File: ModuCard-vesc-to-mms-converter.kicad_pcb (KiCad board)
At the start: 2 copper layers, 60 x 94.5 mm, 42 parts, among them J1 RJ45_LED_Shielded, J2 RJ45_LED_Shielded, J3 Conn_01x04, J4 Conn_01x05, J5 VCC_IN, SW1 SW_DIP_x02, U1 CH334R, Y1 12Mhz

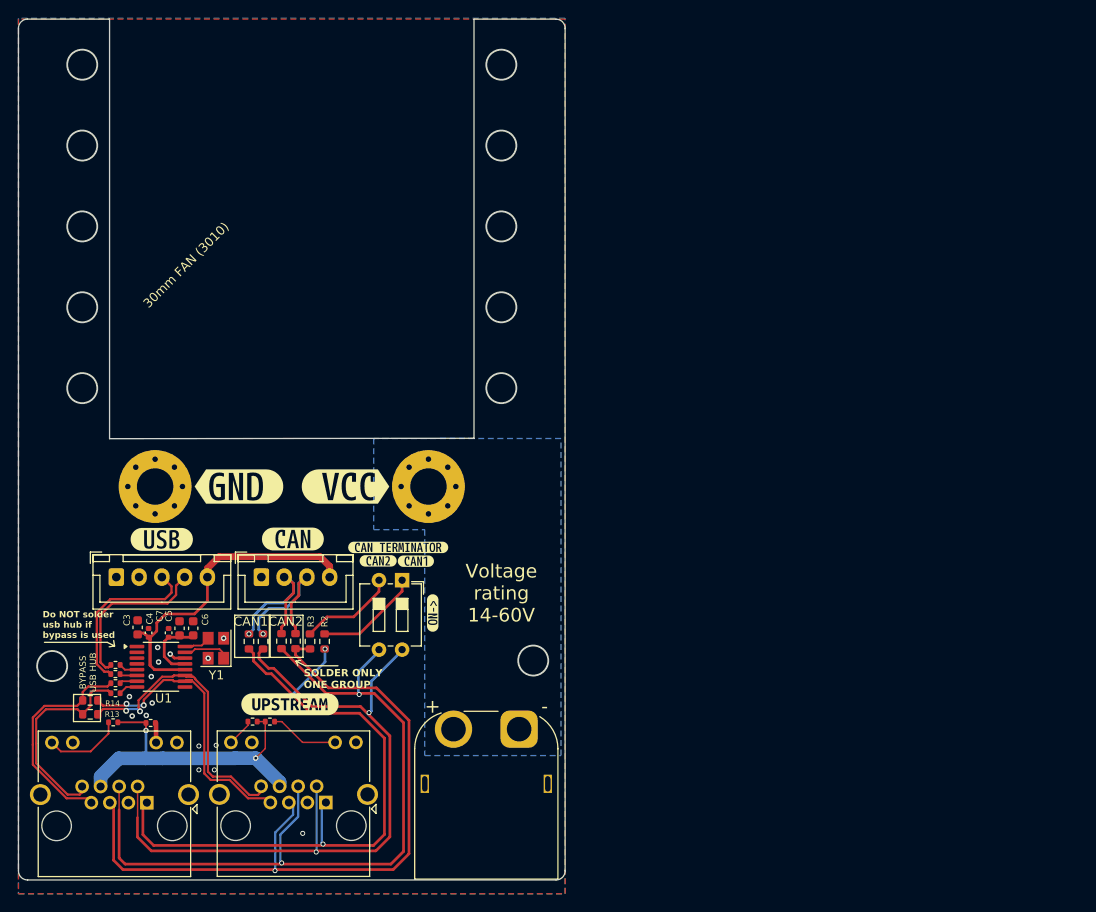
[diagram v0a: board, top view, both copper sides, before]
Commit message: rev v3 tiny
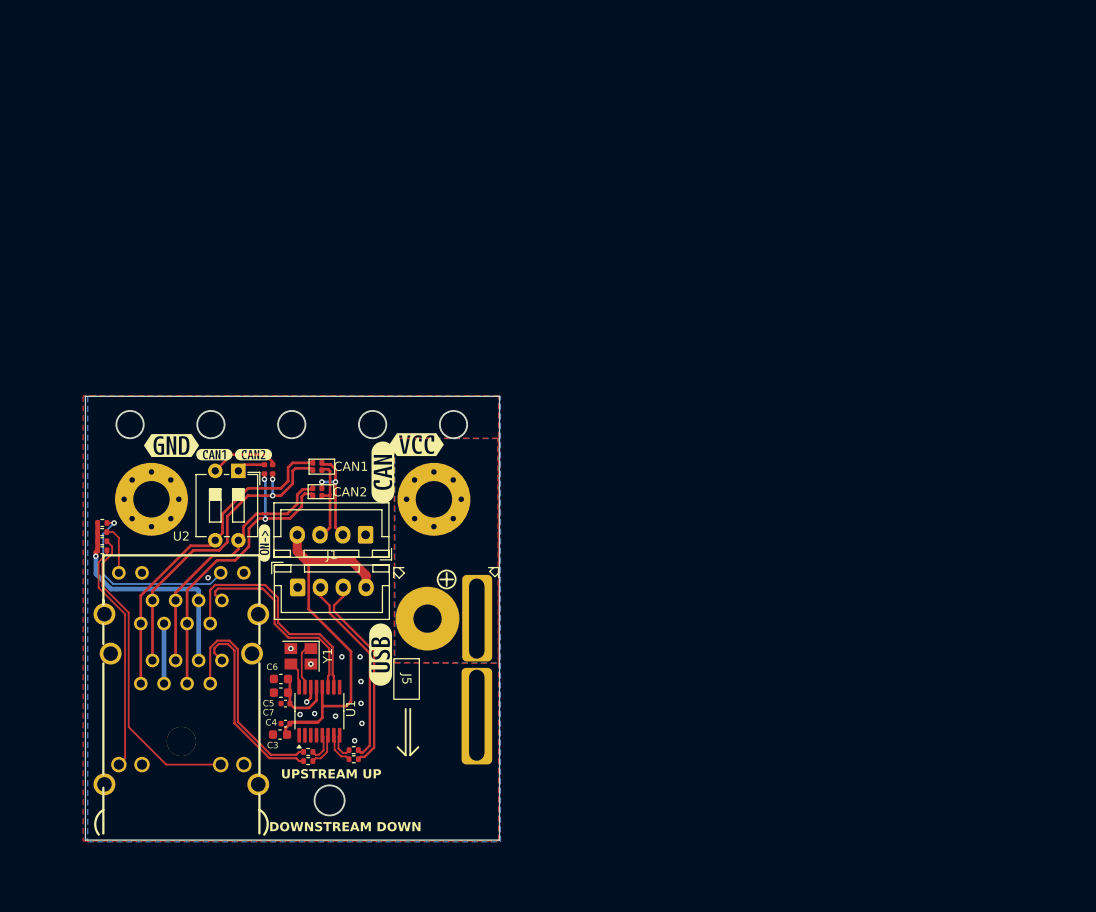
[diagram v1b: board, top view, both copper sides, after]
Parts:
- removed J2: RJ45_LED_Shielded, Connector_RJ:RJ45_Amphenol_RJHSE538X
- removed J4: Conn_01x05, Connector_JST:JST_XH_B5B-XH-A_1x05_P2.50mm_Vertical
- removed R13, R14, R8: 0R, Resistor_SMD:R_0603_1608Metric
- removed R17, R18: 1k, Resistor_SMD:R_0402_1005Metric
- removed R3: 120R, Resistor_SMD:R_0603_1608Metric
- removed kibuzzard-673147F0: G***, kibuzzard-673147F0
- removed kibuzzard-67314807: G***, kibuzzard-67314807
- removed kibuzzard-674E462A: G***, kibuzzard-674E462A
- removed kibuzzard-6754762D: G***, kibuzzard-6754762D
- removed kibuzzard-675D9C67: G***, kibuzzard-675D9C67
- removed kibuzzard-68D8378B: G***, kibuzzard-68D8378B
- removed kibuzzard-68D83794: G***, kibuzzard-68D83794
- added R15: 1k, Resistor_SMD:R_0402_1005Metric, F.Cu at (89.2, 111.3)
- added R16: 1k, Resistor_SMD:R_0402_1005Metric, F.Cu at (89.2, 112.3)
- added R19: 1k, Resistor_SMD:R_0402_1005Metric, F.Cu at (89.2, 109.3)
- added R20: 1k, Resistor_SMD:R_0402_1005Metric, F.Cu at (89.2, 110.3)
- added U2: XDRJ-1609-002, rj45:RJ45-TH_XDRJ-1609-002, F.Cu at (97.9, 126.4)
- added kibuzzard-68DAF865: G***, kibuzzard-68DAF865, F.Cu at (123.7, 100.7)
- added kibuzzard-68DAF86F: G***, kibuzzard-68DAF86F, F.Cu at (96.8, 100.8)
- added kibuzzard-68DB0050: G***, kibuzzard-68DB0050, F.Cu at (120.0, 103.8)
- J1: value RJ45_LED_Shielded -> Conn_01x04; footprint Connector_RJ:RJ45_Amphenol_RJHSE538X -> Connector_JST:JST_XH_B4B-XH-A_1x04_P2.50mm_Vertical
- J5: footprint Connector_AMASS:AMASS_XT60PW-M_1x02_P7.20mm_Horizontal -> lib:XT60-RightAngle-Adapter
- R1, R4: value 1k -> 0Ω; footprint Resistor_SMD:R_0402_1005Metric -> PCM_JLCPCB:R_0402
- R2: value 120R -> 120Ω; footprint Resistor_SMD:R_0603_1608Metric -> PCM_JLCPCB:R_0402
- R5, R6: value 0R -> 0Ω; footprint Resistor_SMD:R_0603_1608Metric -> PCM_JLCPCB:R_0402
- R7: value 0R -> 120Ω; footprint Resistor_SMD:R_0603_1608Metric -> PCM_JLCPCB:R_0402
- moved R4 36.2 mm to (112.8, 102.7), turned to 0 degrees
- moved R1 28.1 mm to (112.8, 103.5)
- moved R11 27.4 mm to (116.8, 135.2), turned to 0 degrees
- moved kibuzzard-674E4620 27.1 mm to (119.8, 123.8), turned to 90 degrees
- moved R12 26.9 mm to (116.8, 134.2), turned to 180 degrees
- moved kibuzzard-675D9C73 25.0 mm to (101.5, 101.8)
- moved J1 23.8 mm to (110.7, 116.4), turned to 0 degrees
- moved R10 23.2 mm to (111.8, 135.4)
- moved R9 23.2 mm to (111.8, 134.4)
- moved SW1 21.6 mm to (104.1, 103.6)
- moved kibuzzard-675D9CCD 20.0 mm to (107.0, 111.5)
- moved R2 19.7 mm to (107.9, 103.4)
- moved C3 19.6 mm to (108.7, 132.5), turned to 0 degrees
- moved R7 19.0 mm to (107.0, 103.4)
- moved U1 18.1 mm to (113.0, 130.0), turned to 90 degrees
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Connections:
- J1 pad 1: /CAN/CAN1- -> GND
- J1 pad 2: /CAN/CAN1+ -> /USB/USB_VESC_D+
- J1 pad 3: GND -> /USB/USB_VESC_D-
- J1 pad 4: /CAN/CAN2- -> +5V
- J5 pad 1: GND -> VCC
- J5 pad 2: VCC -> GND
- R1 pad 1: +12V -> /CAN/CAN1+
- R1 pad 2: Net-(J1-Pad10) -> /CAN/CAN+
- R10 pad 1: /USB/USB_VESC_D+ -> USB_DOWNSTREAM_D+
- R11 pad 2: USB_DOWNSTREAM_D- -> /USB/USB_VESC_D-
- R12 pad 1: USB_DOWNSTREAM_D+ -> /USB/USB_VESC_D+
- R2 pad 1: /CAN/CAN1- -> /CAN/CAN1+
- R4 pad 1: +12V -> /CAN/CAN1-
- R4 pad 2: Net-(J2-Pad12) -> /CAN/CAN-
- R5 pad 1: /CAN/CAN2+ -> /CAN/CAN+
- R5 pad 2: /CAN/CAN+ -> /CAN/CAN2+
- R6 pad 1: /CAN/CAN+ -> /CAN/CAN-
- R6 pad 2: /CAN/CAN1+ -> /CAN/CAN2-
- R7 pad 1: /CAN/CAN2- -> /CAN/CAN2+
- R7 pad 2: /CAN/CAN- -> Net-(R7-Pad2)
- R9 pad 1: /USB/USB_VESC_D- -> USB_DOWNSTREAM_D-
- SW1 pad 1: Net-(R2-Pad2) -> Net-(R7-Pad2)
- SW1 pad 2: Net-(R3-Pad2) -> Net-(R2-Pad2)
- SW1 pad 3: /CAN/CAN2- -> /CAN/CAN1-
- SW1 pad 4: /CAN/CAN1+ -> /CAN/CAN2-
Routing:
- net /CAN/CAN2-: track 86.0 -> 29.5 mm, vias 2 -> 0
- net /CAN/CAN2+: track 80.9 -> 35.3 mm, vias 1 -> 2
- net /CAN/CAN1+: track 80.4 -> 35.7 mm
- net /CAN/CAN1-: track 72.7 -> 36.7 mm, vias 3 -> 0
- net Net-(R15-Pad1): track 0.00 -> 34.1 mm
- net Net-(R16-Pad1): track 0.00 -> 25.4 mm
- net Net-(R19-Pad1): track 0.00 -> 20.8 mm, vias 0 -> 1
- net Net-(R3-Pad2): track 10.7 -> 0.00 mm
- net USB_UPSTREAM_D+: track 33.1 -> 22.5 mm, vias 2 -> 0
- net +12V: track 35.4 -> 25.4 mm, vias 2 -> 1
- net Net-(J2-Pad12): track 8.66 -> 0.00 mm
- net Net-(J1-Pad10): track 7.59 -> 0.00 mm
- net /CAN/CAN+: track 17.1 -> 9.64 mm, vias 1 -> 0
- net GND: track 1.81 -> 8.40 mm, vias 15 -> 13
- net USB_UPSTREAM_D-: track 32.5 -> 26.2 mm, vias 2 -> 0
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- added copper zone on F.Cu, net VCC
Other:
- board size 60 x 94.5 mm -> 45.5 x 48.7 mm
- board text added: "DOWNSTREAM DOWN"
- board text added: "UPSTREAM UP"
- board text removed: "30mm FAN (3010)"
- board text removed: "BYPASS USB HUB"
- board text removed: "Do NOT solder usb hub if bypass is used"
- board text removed: "R13"
- board text removed: "R14"
- board text removed: "SOLDER ONLY ONE GROUP"
- board text removed: "USB BYPASS BLOCK DIAGRAM"
- board text removed: "USB HUB"
- board text removed: "USB IN"
- board text removed: "USB OUT"

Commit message: rev 1
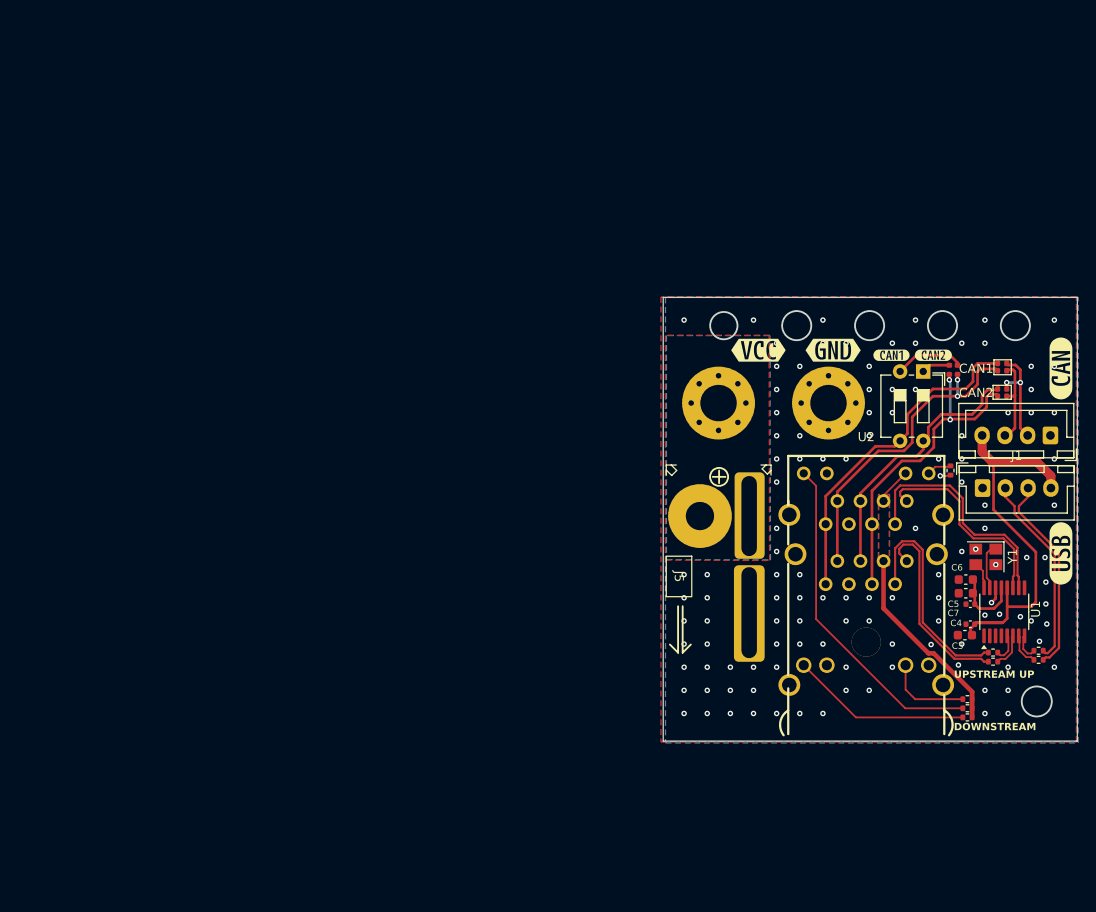
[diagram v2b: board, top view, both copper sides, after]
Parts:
- removed kibuzzard-675D9CCD: G***, kibuzzard-675D9CCD
- moved R20 96.9 mm to (184.2, 129.6), turned to 0 degrees
- moved R16 96.7 mm to (184.2, 130.6), turned to 0 degrees
- moved R15 96.5 mm to (184.2, 128.6), turned to 0 degrees
- moved R19 93.3 mm to (182.3, 103.5), turned to -90 degrees
- moved J3 76.0 mm to (193.3, 99.7)
- moved R7 76.0 mm to (182.2, 92.5)
- moved U1 76.0 mm to (188.2, 119.1)
- moved U2 76.0 mm to (173.0, 115.5)
- moved Y1 76.0 mm to (186.2, 113.0)
- moved C3 76.0 mm to (183.9, 121.6)
- moved R1 76.0 mm to (188.0, 92.6)
- moved R10 76.0 mm to (187.0, 124.5)
- moved R11 76.0 mm to (192.0, 124.3)
- moved R12 76.0 mm to (192.0, 123.3)
- moved R4 76.0 mm to (188.0, 91.8)
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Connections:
- R19 pad 2: +12V -> GND
- U2 pad 21: GND -> Net-(R19-Pad1)
- U2 pad 22: Net-(R19-Pad1) -> +12V
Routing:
- net Net-(R20-Pad1): track 5.43 -> 36.7 mm
- net Net-(R15-Pad1): track 34.1 -> 9.39 mm
- net Net-(R19-Pad1): track 20.8 -> 2.73 mm, vias 1 -> 0
- net GND: track 8.40 -> 2.82 mm, vias 13 -> 122
- net Net-(R16-Pad1): track 25.4 -> 19.8 mm
- net +12V: track 25.4 -> 25.6 mm, vias 1 -> 0
- added copper zone on B.Cu, net +12V
- added copper zone on F.Cu, net +12V
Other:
- outline, holes or cut-outs redrawn
- board text added: "DOWNSTREAM"
- board text removed: "DOWNSTREAM DOWN"
